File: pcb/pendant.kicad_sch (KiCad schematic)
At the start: 246 parts, among them J1 Conn_01x02, J2 USB_B_Micro, U1 ATSAMD21G18A-A, U2 LSM6DS3, U3 XC6206PxxxMR, U4 TP4057

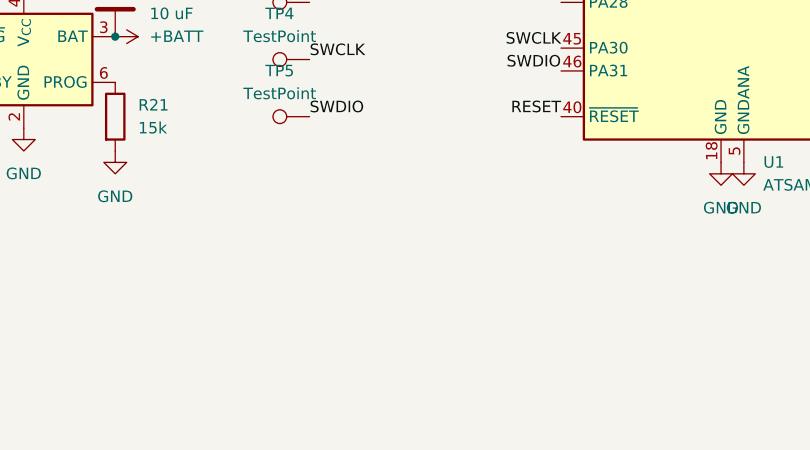
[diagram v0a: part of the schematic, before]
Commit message: Revise PCB
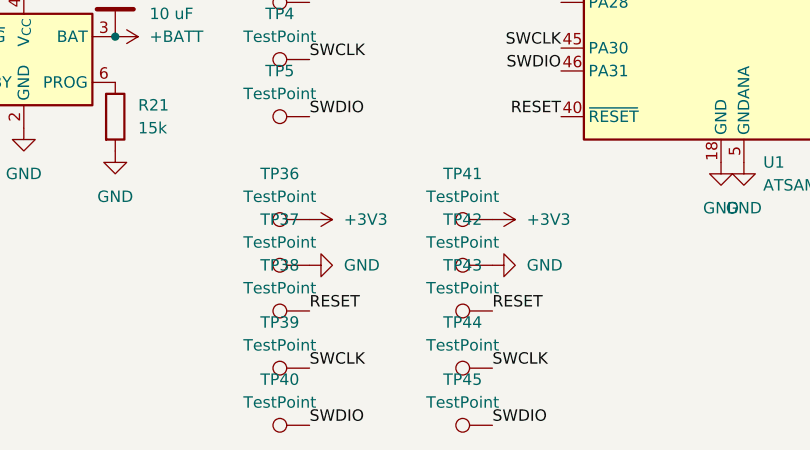
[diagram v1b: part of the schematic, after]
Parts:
- added TP36, TP37, TP38, TP39, TP40: TestPoint, TestPoint:TestPoint_THTPad_D2.0mm_Drill1.0mm, symbol Connector:TestPoint
- added TP41, TP42, TP43, TP44, TP45: TestPoint, TestPoint:TestPoint_Pad_D3.0mm, symbol Connector:TestPoint
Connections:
- net +3V3: now also TP36.1, TP41.1
- net GND: now also TP37.1, TP42.1
- net RESET: now also TP38.1, TP43.1
- net SWCLK: now also TP39.1, TP44.1
- net SWDIO: now also TP40.1, TP45.1

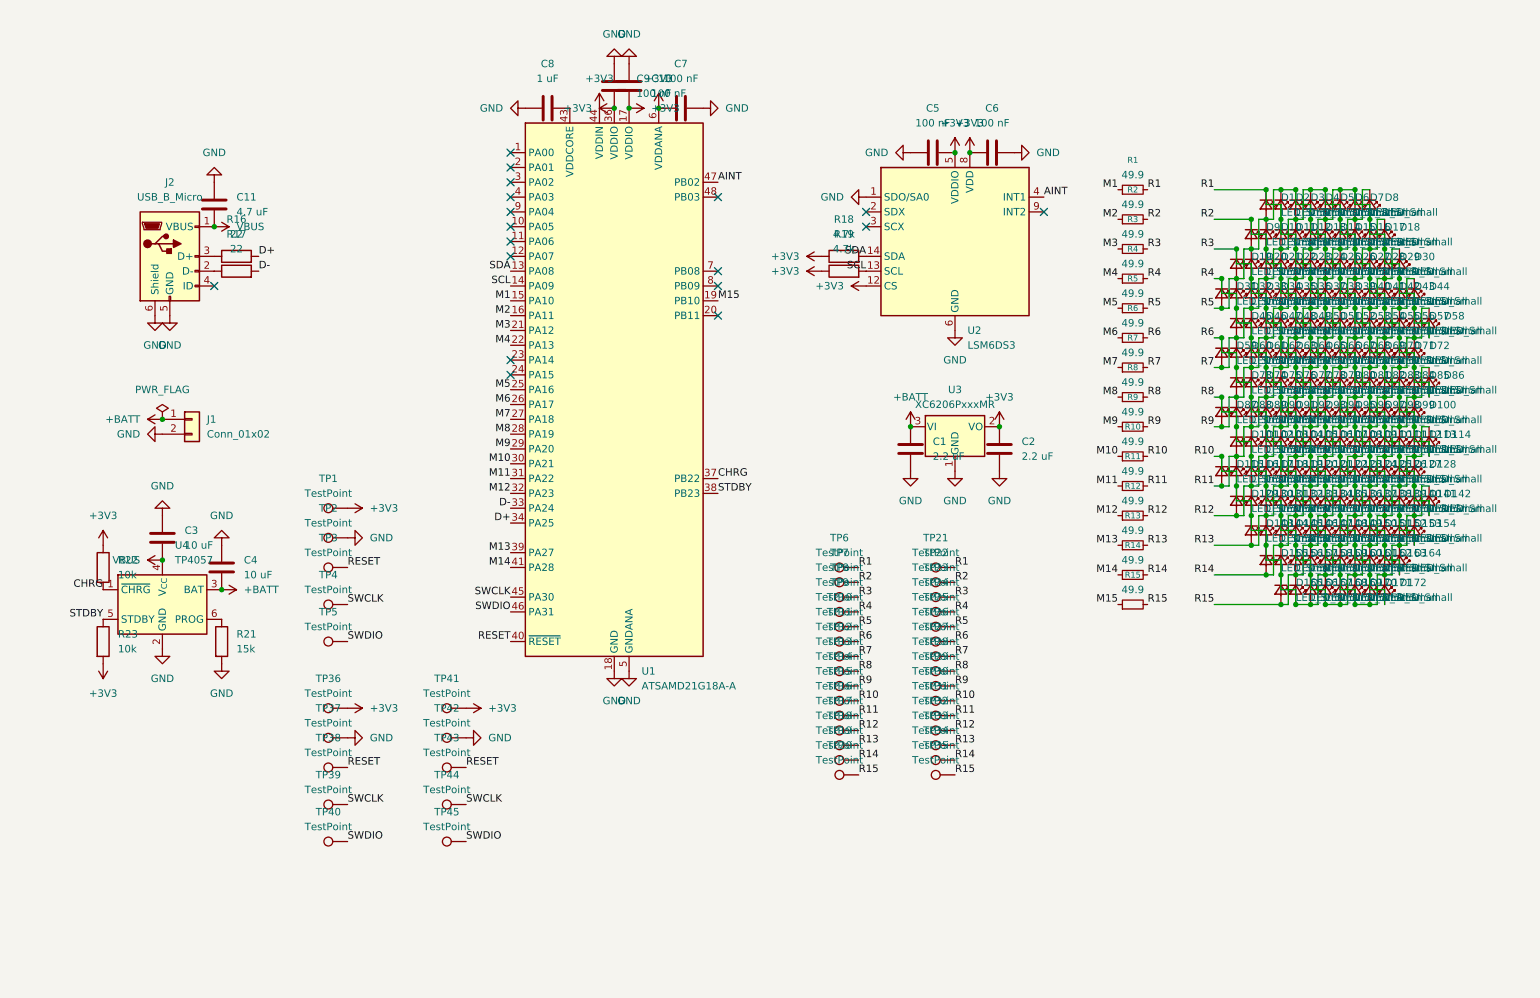
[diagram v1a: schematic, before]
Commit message: Format schematic
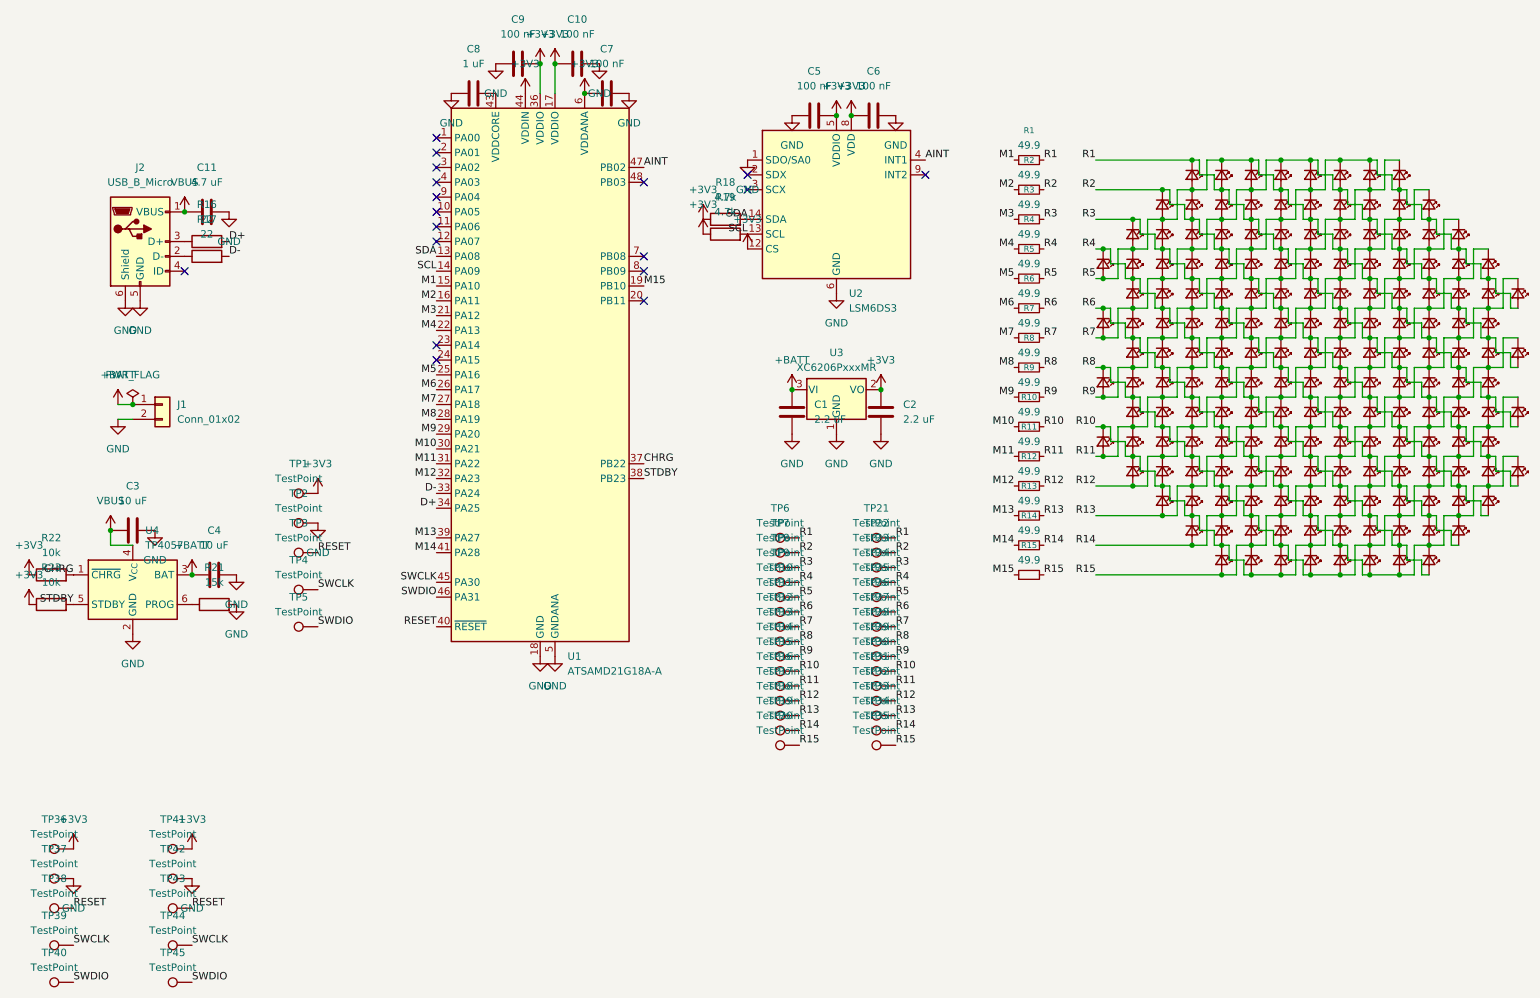
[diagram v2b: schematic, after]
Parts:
- D1, D10, D100, D101, D102, D103, D104, D105, D106, D107, D108, D109, D11, D110, D111, D112, D113, D114, D115, D116, D117, D118, D119, D12, D120, D121, D122, D123, D124, D125, D126, D127, D128, D129, D13, D130, D131, D132, D133, D134, D135, D136, D137, D138, D139, D14, D140, D141, D142, D143, D144, D145, D146, D147, D148, D149, D15, D150, D151, D152, D153, D154, D155, D156, D157, D158, D159, D16, D160, D161, D162, D163, D164, D165, D166, D167, D168, D169, D17, D170, D171, D172, D18, D19, D2, D20, D21, D22, D23, D24, D25, D26, D27, D28, D29, D3, D30, D31, D32, D33, D34, D35, D36, D37, D38, D39, D4, D40, D41, D42, D43, D44, D45, D46, D47, D48, D49, D5, D50, D51, D52, D53, D54, D55, D56, D57, D58, D59, D6, D60, D61, D62, D63, D64, D65, D66, D67, D68, D69, D7, D70, D71, D72, D73, D74, D75, D76, D77, D78, D79, D8, D80, D81, D82, D83, D84, D85, D86, D87, D88, D89, D9, D90, D91, D92, D93, D94, D95, D96, D97, D98, D99: symbol Device:LED_Small -> Project:LED_Small
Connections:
- net +3V3: now also C10.1, R23.1; no longer C10.2, R23.2
- net +BATT: now also C4.2; no longer C4.1
- net GND: now also C10.2, C11.2, C3.1, C4.1; no longer C10.1, C11.1, C3.2, C4.2
- net STDBY: now also R23.2; no longer R23.1
- net VBUS: now also C11.1, C3.2; no longer C11.2, C3.1
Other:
- moved on the sheet: C1, C10, C11, C2, C3, C4, C5, C6, C7, C8, C9, J1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
